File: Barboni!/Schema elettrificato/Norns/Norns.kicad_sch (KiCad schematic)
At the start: 30 parts, among them J1 Power Supply, J2 RPi_GPIO, J3 Display, J4 Encoders, J5 MIDI_Din, J6 MIDI_Din, Q1 S8550, Q2 2N7000, Q3 2N7000, U1 7404, U2 6N138

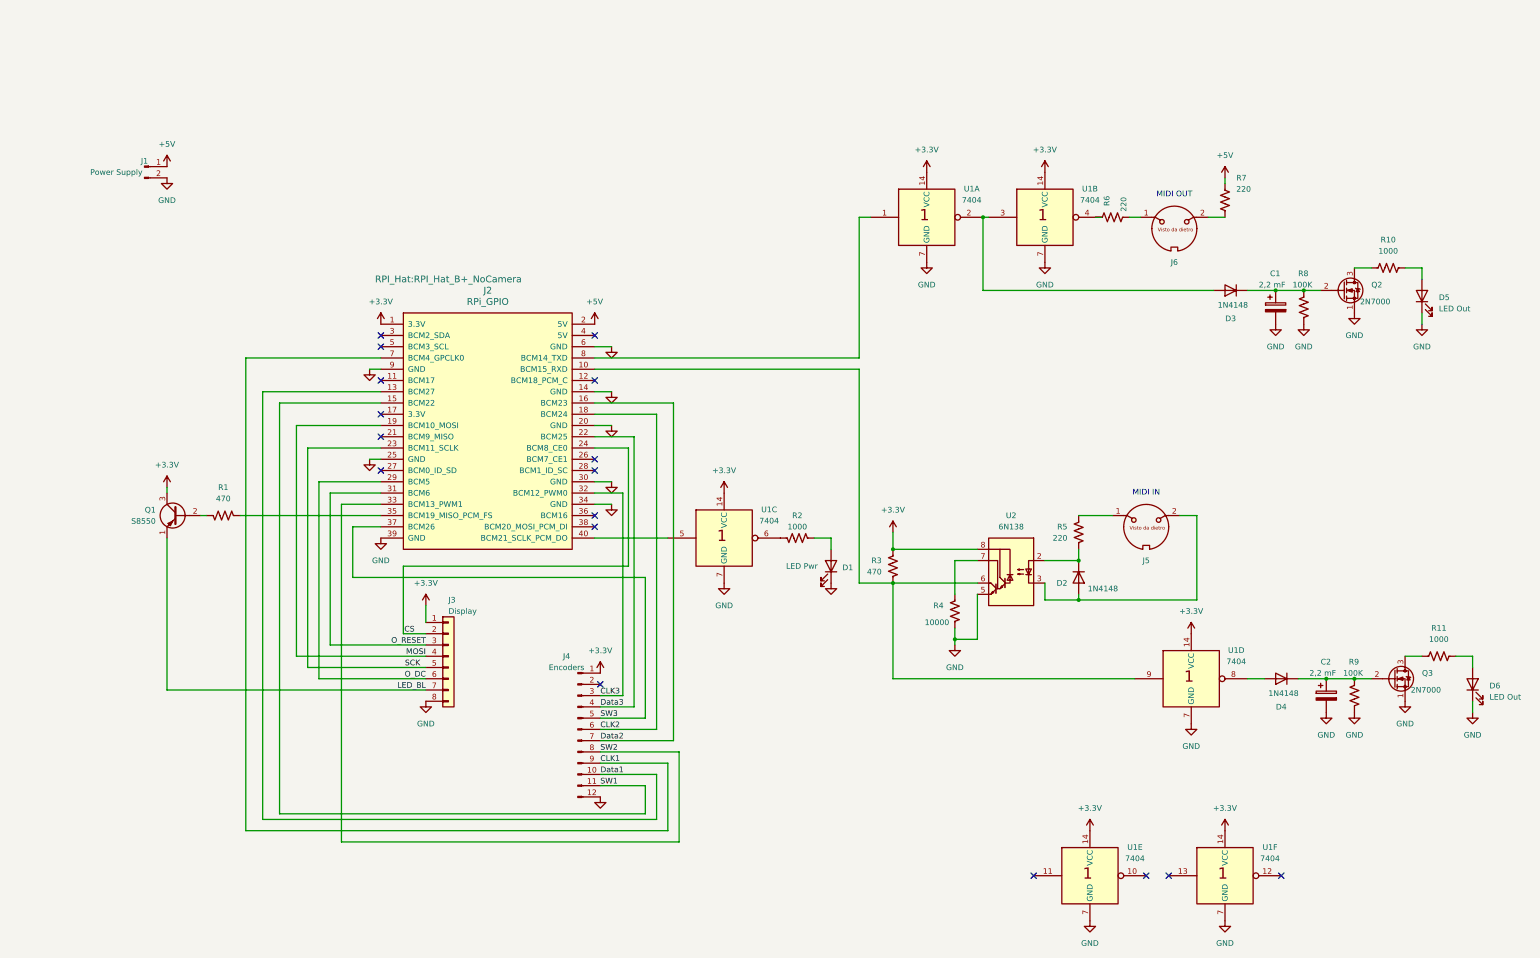
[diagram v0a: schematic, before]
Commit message: a
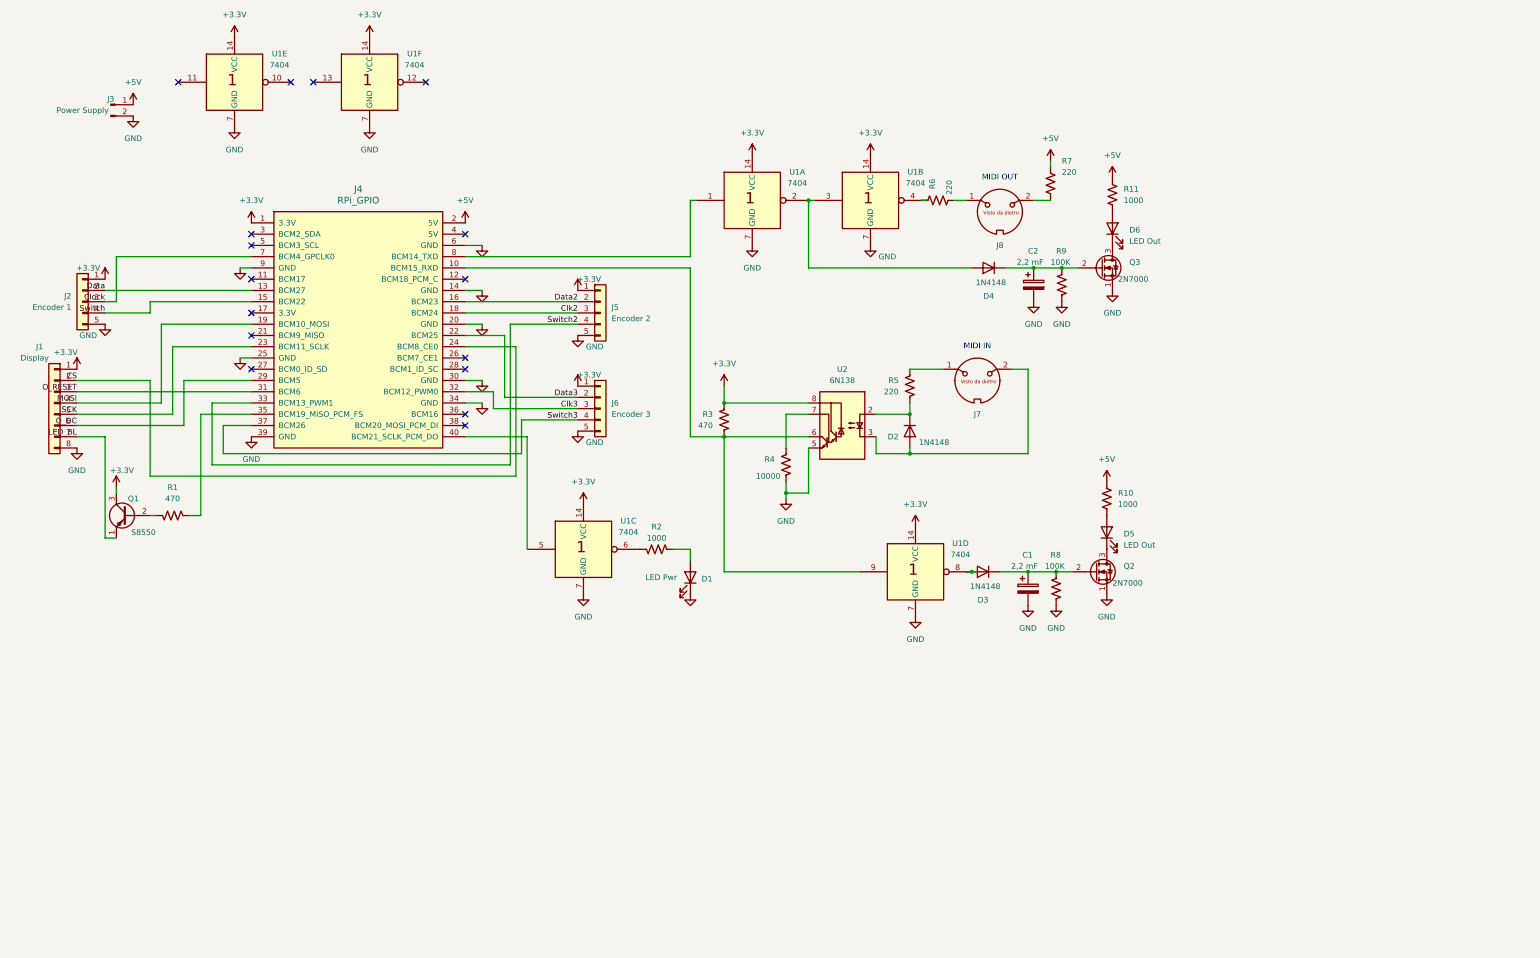
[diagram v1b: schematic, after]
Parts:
- removed J3: Display, Connector_JST:JST_EH_B8B-EH-A_1x08_P2.50mm_Vertical, symbol Connector_Generic:Conn_01x08
- removed J4: Encoders, Connector_JST:JST_EH_B12B-EH-A_1x12_P2.50mm_Vertical, symbol Connector:Conn_01x12_Pin
- added J1: Display, Connector_JST:JST_EH_B8B-EH-A_1x08_P2.50mm_Vertical, symbol Connector_Generic:Conn_01x08
- added J2: Encoder 1, Connector_JST:JST_EH_B5B-EH-A_1x05_P2.50mm_Vertical, symbol Connector_Generic:Conn_01x05
- added J5: Encoder 2, Connector_JST:JST_EH_B5B-EH-A_1x05_P2.50mm_Vertical, symbol Connector_Generic:Conn_01x05
- added J6: Encoder 3, Connector_JST:JST_EH_B5B-EH-A_1x05_P2.50mm_Vertical, symbol Connector_Generic:Conn_01x05
- renumbered C2 to C1, C1 to C2, D4 to D3, D3 to D4, D6 to D5, D5 to D6, J1 to J3, J2 to J4, J5 to J7, J6 to J8, Q3 to Q2, Q2 to Q3, R11 to R10, R10 to R11, R9 to R8, R8 to R9
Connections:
- net +3.3V: now also J1.1 (Pin_1), J2.1 (Pin_1), J5.1 (Pin_1), J6.1 (Pin_1)
- net +5V: now also R10.2, R11.2
- net CS: now also J1.2 (Pin_2)
- net Data2: now also J5.2 (Pin_2)
- net Data3: now also J6.2 (Pin_2)
- net GND: now also J1.8 (Pin_8), J2.5 (Pin_5), J5.5 (Pin_5), J6.5 (Pin_5); no longer D5.1 (K), D6.1 (K)
- net LED_BL: now also J1.7 (Pin_7)
- net MOSI: now also J1.4 (Pin_4)
- net O_DC: now also J1.6 (Pin_6)
- net O_RESET: now also J1.3 (Pin_3)
- net SCK: now also J1.5 (Pin_5)
- net at Q2.3 (D): now also D5.1 (K); no longer R10.1
- net at D5.2 (A): now also R10.1; no longer R10.2
- net at D6.2 (A): now also R11.1; no longer R11.2
- net at Q3.3 (D): now also D6.1 (K); no longer R11.1
- net CLK1 renamed Clock
- net Clock: now also J2.3 (Pin_3)
- net CLK2 renamed Clk2
- net Clk2: now also J5.3 (Pin_3)
- net CLK3 renamed Clk3
- net Clk3: now also J6.3 (Pin_3)
- net Data1 renamed Data
- net Data: now also J2.2 (Pin_2)
- net SW1 renamed Switch
- net Switch: now also J2.4 (Pin_4)
- net SW2 renamed Switch2
- net Switch2: now also J5.4 (Pin_4)
- net SW3 renamed Switch3
- net Switch3: now also J6.4 (Pin_4)
- no-connect marks 17 -> 16
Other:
- moved on the sheet: C1, C2, D1, D2, D3, D4, D5, D6, J3, J4, J7, J8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
